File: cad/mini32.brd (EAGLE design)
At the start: 63 x 35 mm, 52 parts, among them CN1 MICROSDPLAIN, J1 HEADER-5X1, Q1 MOSFETSOT-23, SW2 SWITCHKMR211, SW3 SWITCHKMR211, U1 STM32F411/48, U2 MPU-9150, U3 ADP5062, U4 MCP1824, X1 XTAL32X15, X2 XTAL32X15

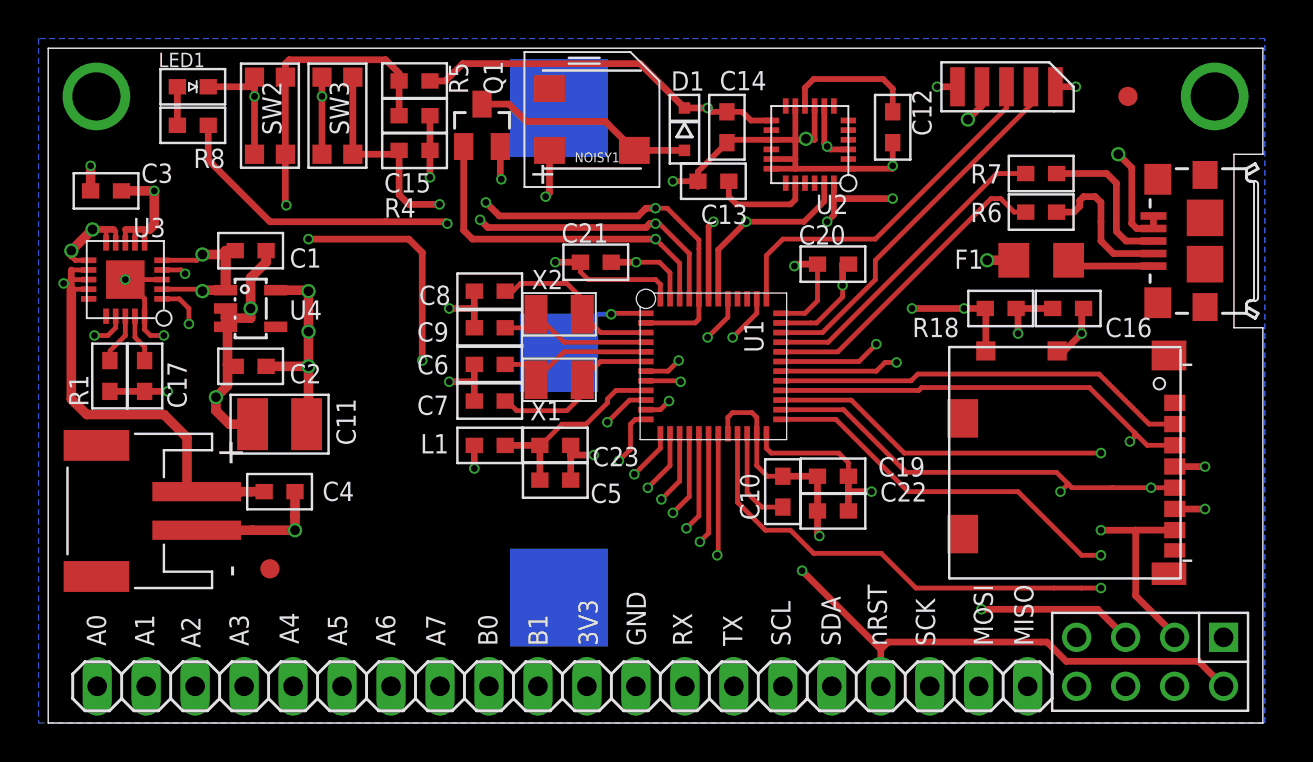
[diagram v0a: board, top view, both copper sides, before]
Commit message: ok
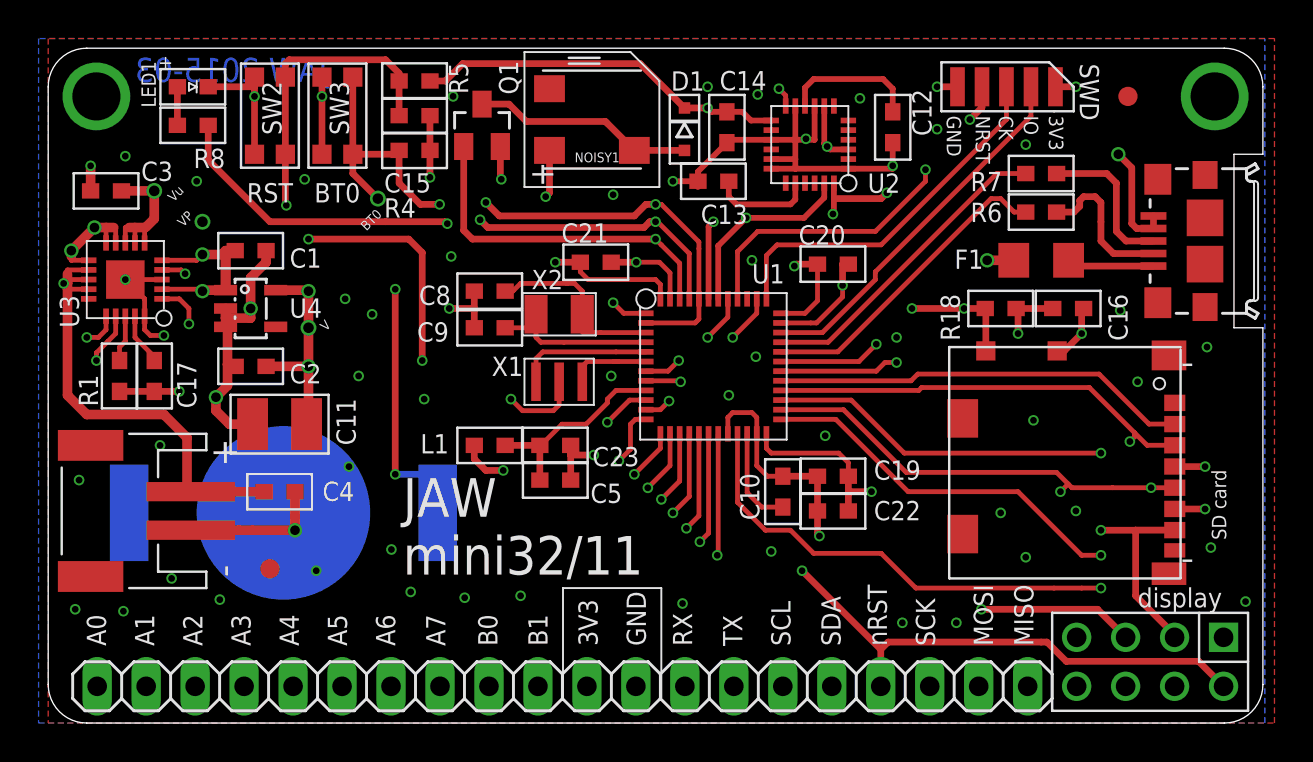
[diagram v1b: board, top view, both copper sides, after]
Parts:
- removed C6, C7: (no value), jaw:SMD0603
- removed U$1: (no value), adafruit:CR2032-SMD
- added B1: BATTERY-CR2016, jaw:CR1216
- added U$4: ROBOTMAN-LOGO, jaw:ROBOTMAN-LOGO
- C12: value (none) -> 0.1u
- C13: value (none) -> 2.2n
- C14: value (none) -> .1u
- C17: value (none) -> 10n
- C8, C9: value (none) -> 5p
- R1: value (none) -> 10k
- R8: value (none) -> 470
- X1: value XTAL32X15 -> 12MHz; device jaw:XTAL-32X15 -> jaw:RESONATOR-CSTCE
- X2: value XTAL32X15 -> 32k768
- moved C17 0.50 mm to (5.50, 18.0)
- moved R1 0.50 mm to (3.70, 18.0)
- moved CN3 0.30 mm to (3.70, 11.0)
- moved X1 0.10 mm to (26.5, 17.7)
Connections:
- removed net N$29: U1.P40
- new net IMUINT: U1.P40, U2.12
- net BATSTAT: now also U3.16
- net GND: now also B1.MINUS, X1.2; no longer C6.1, C7.1, U$1.+$2
- net N$12: now also X1.1; no longer C6.2, X1.P$1
- net N$13: now also X1.3; no longer C7.2, X1.P$2
- net N$21: now also B1.PLUS1, B1.PLUS2; no longer U$1.-
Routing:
- net IMUINT: track 0.00 -> 24.7 mm, vias 0 -> 2
- net N$21: track 5.36 -> 27.3 mm, vias 1 -> 3
- net BATSTAT: track 22.1 -> 39.6 mm, vias 1 -> 2
- net N$13: track 9.03 -> 4.20 mm
- net BOOT0: track 32.7 -> 35.2 mm, vias 3 -> 4
- net VP: track 16.9 -> 19.0 mm, vias 4 -> 5
- net NRST: track 130.0 -> 128.3 mm
- net N$12: track 8.40 -> 7.04 mm
- net VCC: track 69.5 -> 70.7 mm
- net GND: track 110.6 -> 111.8 mm, vias 24 -> 72
- net I2CDA: track 92.6 -> 93.3 mm
- net N$15: track 8.99 -> 9.75 mm
- net VBAT: track 33.1 -> 33.8 mm
- net I2CCL: track 90.8 -> 90.1 mm
- added copper zone on layer 1, net GND
- added copper zone on layer 15, net GND
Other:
- outline, holes or cut-outs redrawn
- board text added: "+"
- board text added: "BT0"
- board text added: "CK"
- board text added: "IO"
- board text added: "JAW 2015-03"
- board text added: "JAW mini32/11"
- board text added: "NRST"
- board text added: "Pb"
- board text added: "RST"
- board text added: "SD card"
- board text added: "SWD"
- board text added: "V"
- board text added: "VP"
- board text added: "Vu"
- board text added: "battery - CR1216"
- board text added: "display"
- board text added: "mini32/11 Rev. 0"
- board text added: "www.tcp4me.com"
